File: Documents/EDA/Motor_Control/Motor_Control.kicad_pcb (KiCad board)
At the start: 2 copper layers, 68 x 79 mm, 26 parts, among them J1 - Power +, J2 Barrel_Jack, J3 Pipette, J4 R Home, J5 Z Home, J6 EXP, M1 R, M2 Z, U1 ESP32-DEVKITC-32D

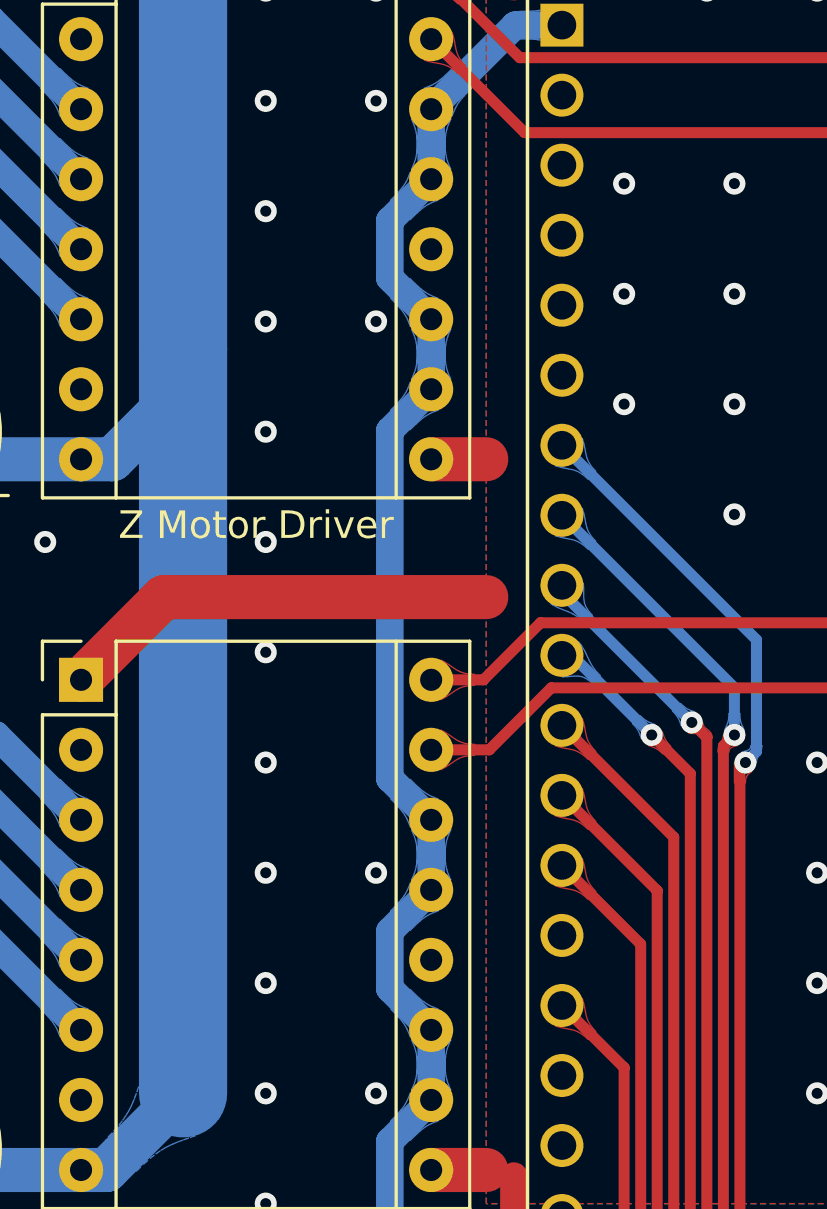
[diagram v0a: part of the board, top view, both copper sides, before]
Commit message: ring light
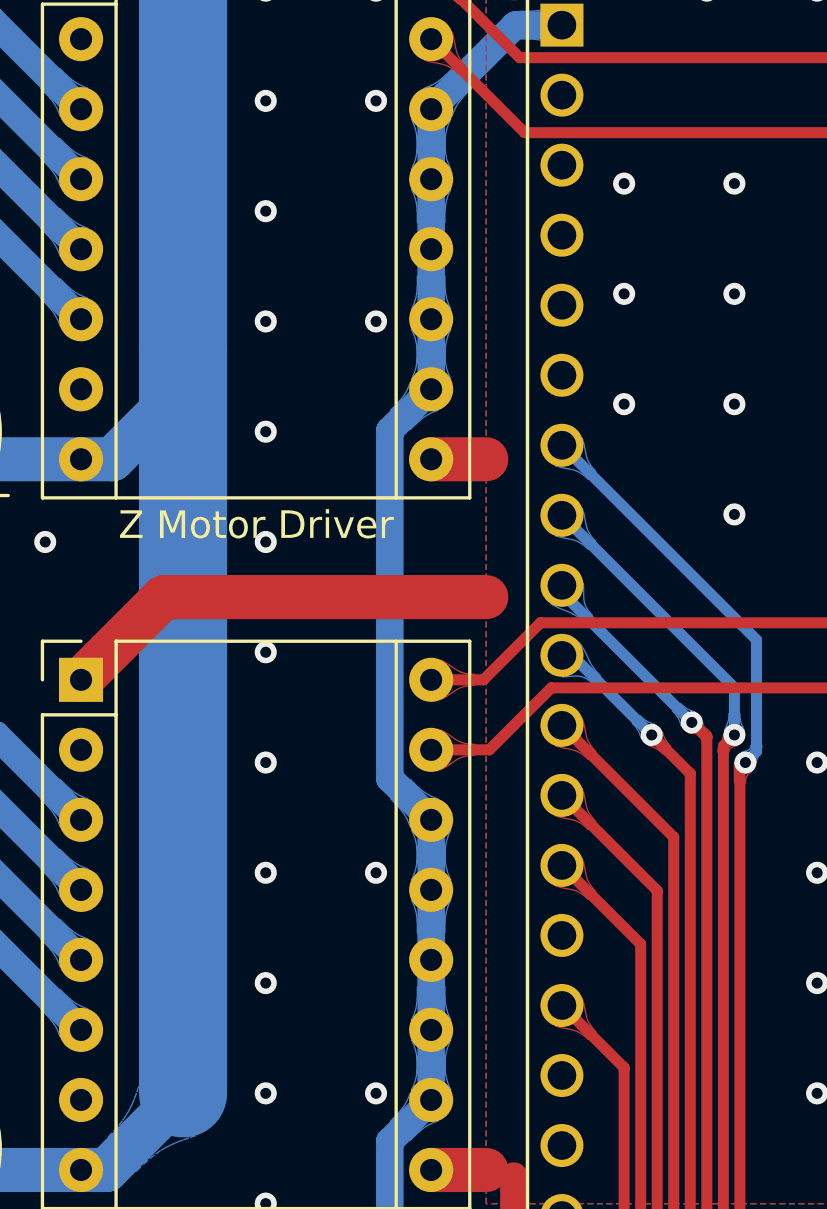
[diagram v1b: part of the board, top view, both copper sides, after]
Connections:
- A1 pad 12: Net-(A1-Pad12) -> +3V3
- A2 pad 12: Net-(A2-Pad12) -> +3V3
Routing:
- net +3V3: track 55.7 -> 53.2 mm
